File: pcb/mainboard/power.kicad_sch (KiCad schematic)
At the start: 45 parts, among them SW101 SW_Push, U101 PCA9450BHN, U102 BQ27441-G1, U103 BQ24072RGT, Y101 32.768K

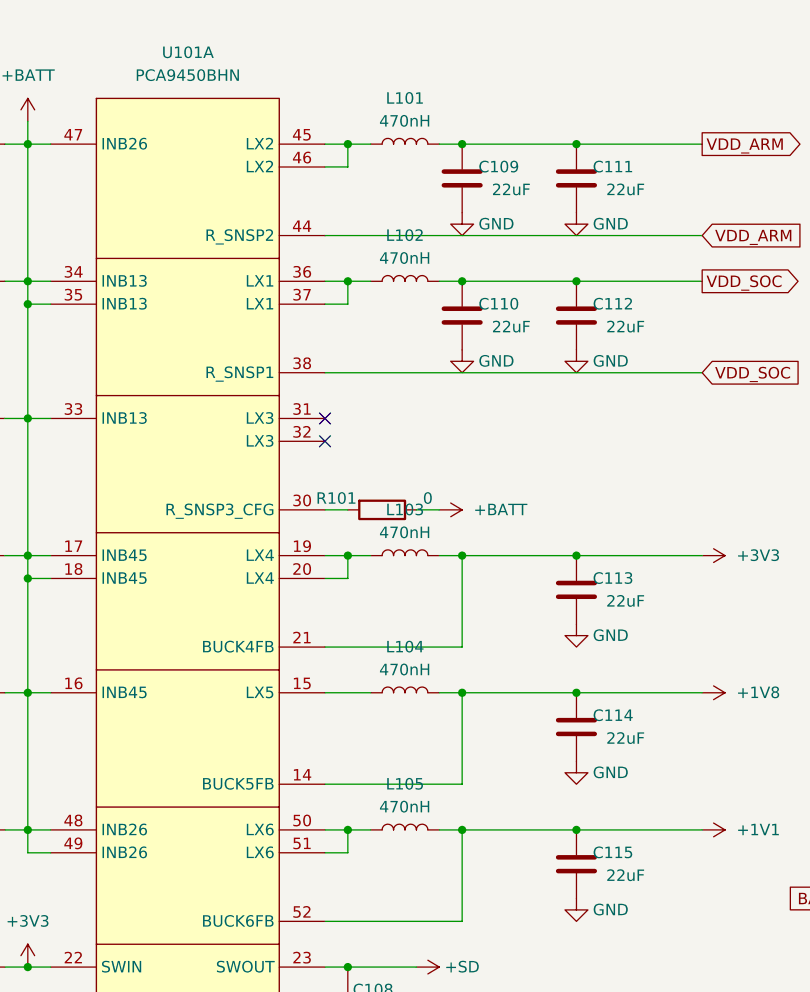
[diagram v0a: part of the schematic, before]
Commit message: Keypad bugfix, pulling in submodules
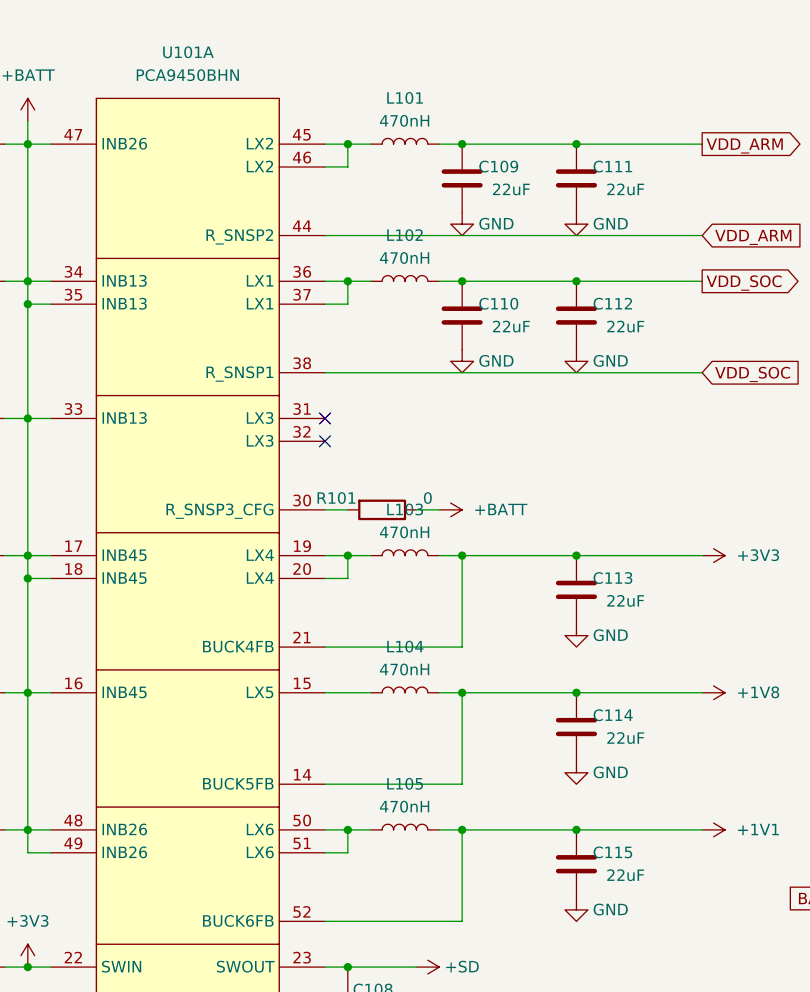
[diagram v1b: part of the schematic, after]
